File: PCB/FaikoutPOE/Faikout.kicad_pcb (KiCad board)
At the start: 2 copper layers, 58 x 65 mm, 85 parts, among them J1 RJ45_LED, J2 S21, J5 Reset, J7 TC2030-USB-NL-DS, M3 Ag97012-FL, P1 Square, Q1 BSS138PS, U1 KSZ8851SNL, U2 ESP32-S3-MINI-1, U3 TCMT1100, U4 TPS62933, U5 TCMT1100, Y1 Crystal_GND24

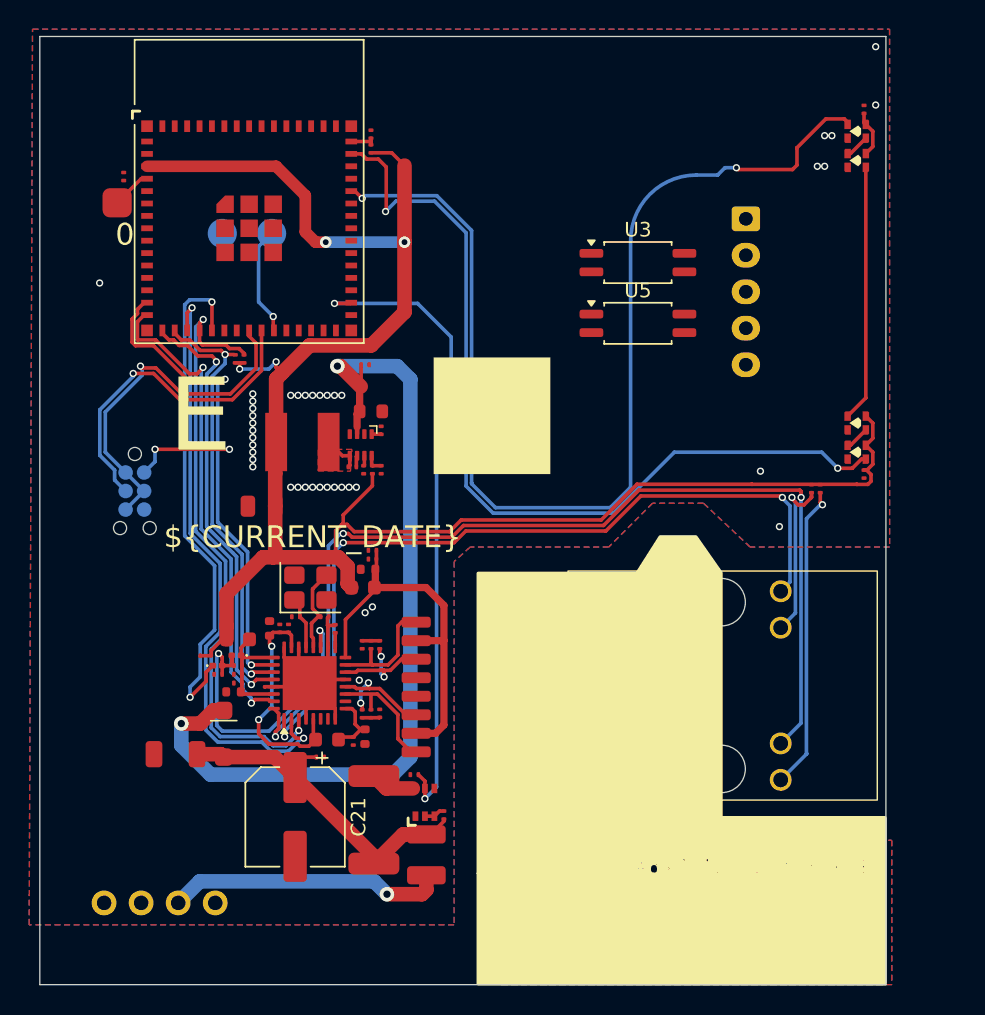
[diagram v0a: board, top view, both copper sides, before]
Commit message: Started on POE
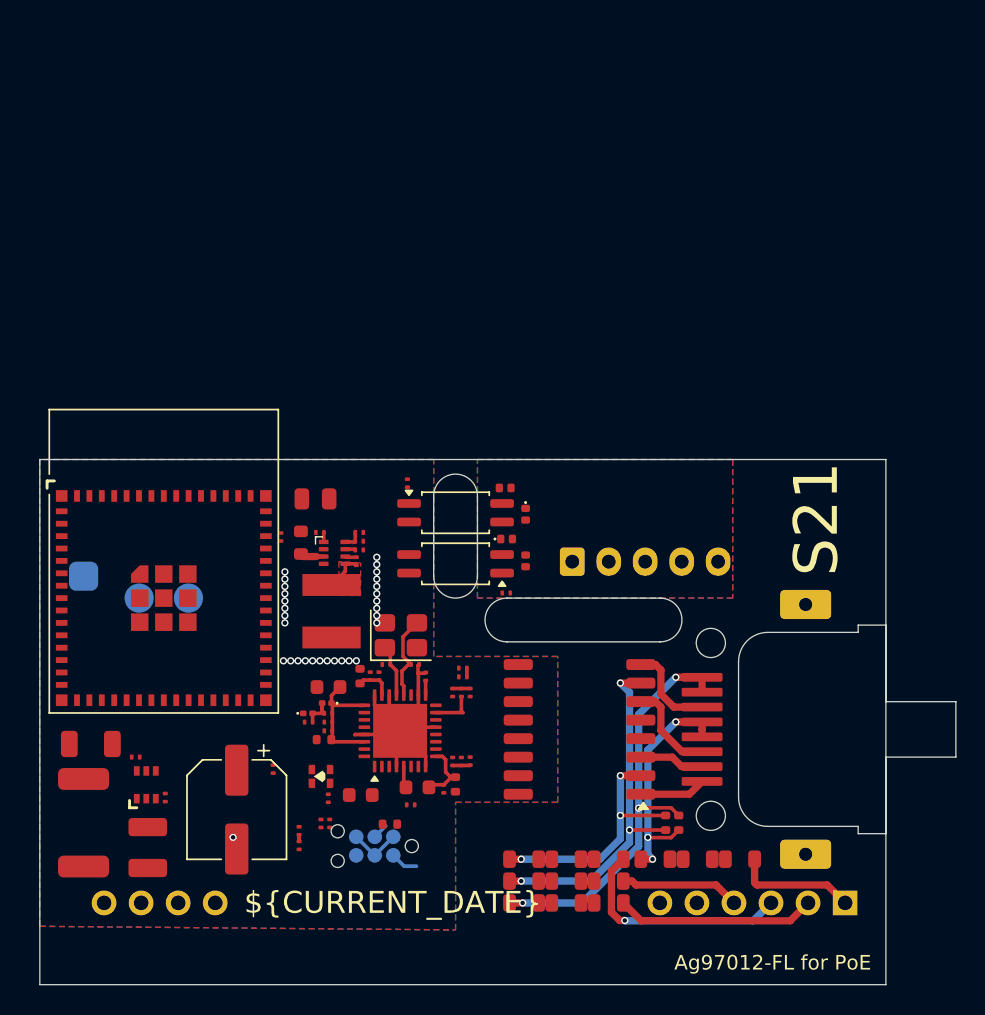
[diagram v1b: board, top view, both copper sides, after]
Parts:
- removed C35: 100nF, RevK:C_0201
- removed D21: DKS34, RevK:D_SOD-123FL
- added D3: ~, RevK:DFN1006-2L, F.Cu at (131.9, 66.0)
- D5: value XL-1615RGBC-2812B -> ~; footprint RevK:SMD1615-Side -> RevK:DFN1006-2L
- D6, D7: value XL-1615RGBC-2812B -> D; footprint RevK:SMD1615-Side -> RevK:D_0402
- J1: footprint RevK:HC-WK88-H21-DKH -> RevK:RC01516
- P1: moved to B.Cu
- R6: value 49R9 -> 10k
- moved C36 48.0 mm to (117.8, 89.5)
- moved R9 48.0 mm to (117.8, 90.5)
- moved C34 42.9 mm to (119.8, 87.2)
- moved D4 42.9 mm to (119.3, 85.7)
- moved C17 41.9 mm to (116.0, 85.2)
- moved D6 35.3 mm to (132.0, 69.5)
- moved D7 34.7 mm to (133.3, 67.8), turned to -90 degrees
- moved R18 32.4 mm to (119.9, 89.0)
- moved R19 32.4 mm to (119.3, 89.0)
- moved J7 29.4 mm to (123.0, 90.5), turned to 180 degrees
- moved R5 27.7 mm to (125.2, 65.6)
- moved J2 26.3 mm to (136.5, 71.0), turned to 0 degrees
- moved U2 26.0 mm to (108.5, 73.5)
- moved P1 25.7 mm to (103.0, 72.0), turned to 180 degrees
- moved J5 25.6 mm to (108.5, 73.5)
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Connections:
- C29 pad 1: VDC -> POE
- C30 pad 1: VDC -> POE
- D4 pad 2: LED -> LEDO
- D4 pad 4: Net-(D4-O) -> LEDI
- D5 pad 1: GND -> S21GND
- D5 pad 2: Net-(D4-O) -> S21RX
- D6 pad 1: GND -> S21RX
- D6 pad 2: Net-(D5-O) -> Net-(D6-A)
- D7 pad 1: GND -> S21TX
- D7 pad 2: Net-(D6-O) -> Net-(D6-A)
- J2 pad 1: unconnected-(J2-Pin_1-Pad1) -> S215V
- J2 pad 2: unconnected-(J2-Pin_2-Pad2) -> S21RX
- J2 pad 3: unconnected-(J2-Pin_3-Pad3) -> S21TX
- J2 pad 5: unconnected-(J2-Pin_5-Pad5) -> S21GND
- R5 pad 2: Net-(J1-Pad11) -> Net-(R5-Pad2)
- R6 pad 1: +3.3V -> S215V
- R6 pad 2: Net-(J1-Pad9) -> Net-(D6-A)
- U1 pad 1: LED0 -> unconnected-(U1-LED0-Pad1)
- U1 pad 32: LED1 -> unconnected-(U1-LED1-Pad32)
- U2 pad 27: unconnected-(U2-GPIO47-Pad27) -> LEDO
- U2 pad 28: unconnected-(U2-GPIO33-Pad28) -> LEDI
- U2 pad 29: unconnected-(U2-GPIO34-Pad29) -> RX
- U2 pad 30: unconnected-(U2-GPIO48-Pad30) -> TX
- U2 pad 41: LEDI -> unconnected-(U2-GPIO45-Pad41)
- U2 pad 44: LED -> unconnected-(U2-GPIO46-Pad44)
- U3 pad 1: unconnected-(U3-Pad1) -> Net-(R5-Pad2)
- U3 pad 2: unconnected-(U3-Pad2) -> TX
- U3 pad 3: unconnected-(U3-Pad3) -> S21GND
- U3 pad 4: unconnected-(U3-Pad4) -> S21TX
- U4 pad 3: VDC -> POE
- U5 pad 1: unconnected-(U5-Pad1) -> S215V
- U5 pad 2: unconnected-(U5-Pad2) -> S21RX
- U5 pad 3: unconnected-(U5-Pad3) -> GND
- U5 pad 4: unconnected-(U5-Pad4) -> RX
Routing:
- net +3.3V: track 132.2 -> 0.00 mm, vias 4 -> 0
- net LEDI: track 75.8 -> 0.00 mm, vias 2 -> 0
- net LED1: track 68.8 -> 0.00 mm, vias 3 -> 0
- net VDC: track 61.0 -> 0.00 mm, vias 2 -> 0
- net LED: track 60.5 -> 0.00 mm, vias 2 -> 0
- net LED0: track 54.6 -> 0.00 mm, vias 3 -> 0
- net POELOAD: track 44.4 -> 0.00 mm, vias 2 -> 0
- net INTR: track 42.4 -> 0.00 mm, vias 2 -> 0
- net PME: track 41.6 -> 0.00 mm, vias 2 -> 0
- net ETHRST: track 35.3 -> 0.00 mm, vias 2 -> 0
- net SI: track 33.9 -> 0.00 mm, vias 2 -> 0
- net CSN: track 33.3 -> 0.00 mm, vias 2 -> 0
- net SCLK: track 30.1 -> 0.00 mm, vias 2 -> 0
- net SO: track 30.0 -> 0.00 mm, vias 2 -> 0
- net VDDA3V3: track 25.7 -> 0.60 mm
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- added copper zone on B.Cu, net S21GND
- added copper zone on F.Cu, net S21GND
- removed copper zone on B.Cu, net Net-(J1-SH-Pad13)
- removed copper zone on F.Cu, net Net-(J1-SH-Pad13)
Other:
- board size 58 x 65 mm -> 58 x 36 mm
- board text added: "Faikout ${CURRENT_DATE}"
- board text added: "S21"
- board text removed: "10 11 12 13 14 15 16 36 45 46"
- board text removed: "CSN MOSI SCLK MISO PME INTR ETHRST POELOAD LEDI LED"
- board text removed: "EnvLED2 ${CURRENT_DATE}"
- board text removed: "H"
- board text removed: "T3902"
- board text removed: "U"
